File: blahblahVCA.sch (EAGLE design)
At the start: 29 parts, among them IC1 CA3080D, IC2 RC4558D, IC3 CA3130D, Q1 BCM847DS

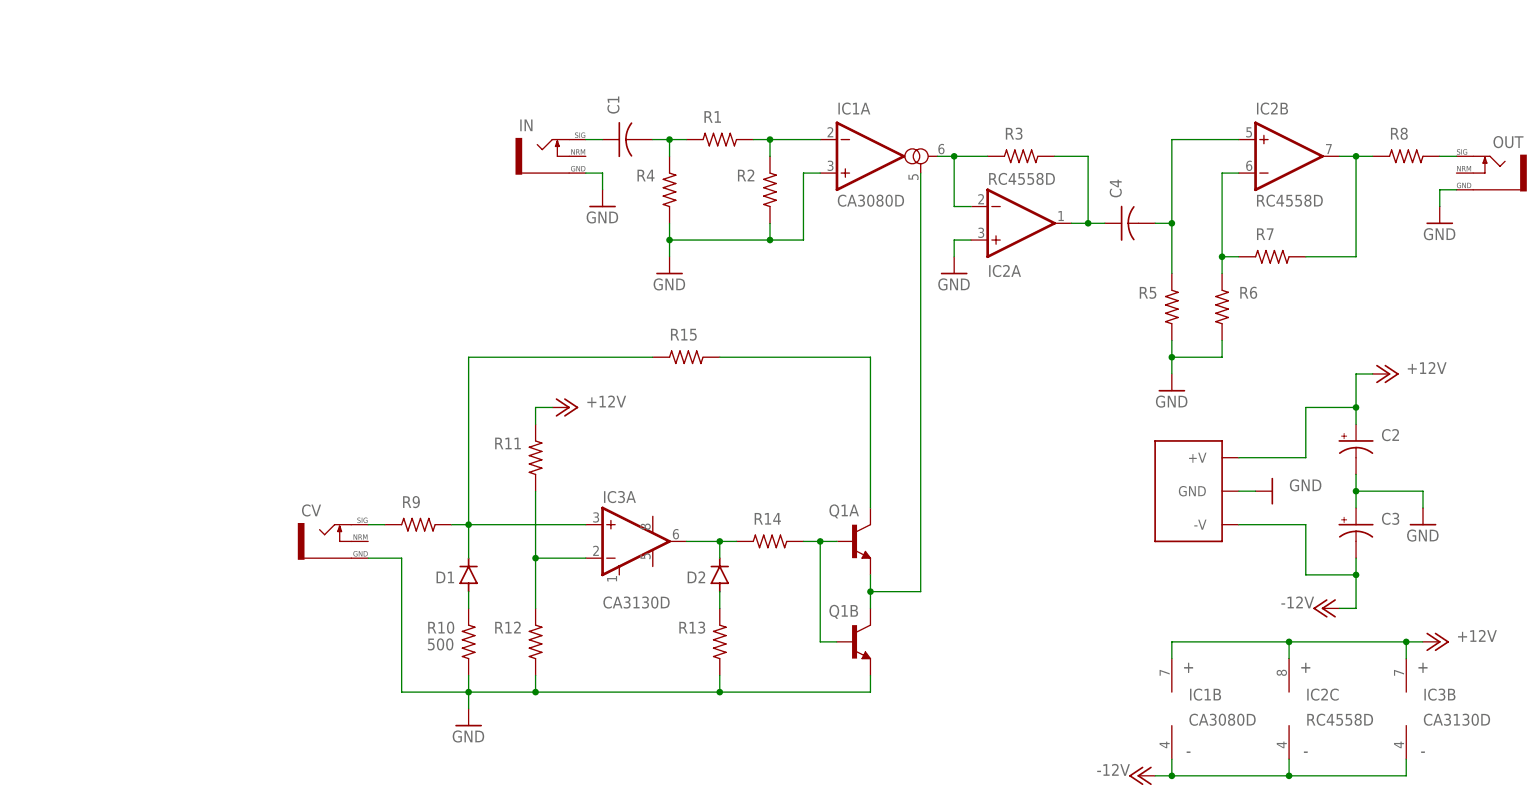
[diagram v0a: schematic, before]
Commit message: Add files via upload
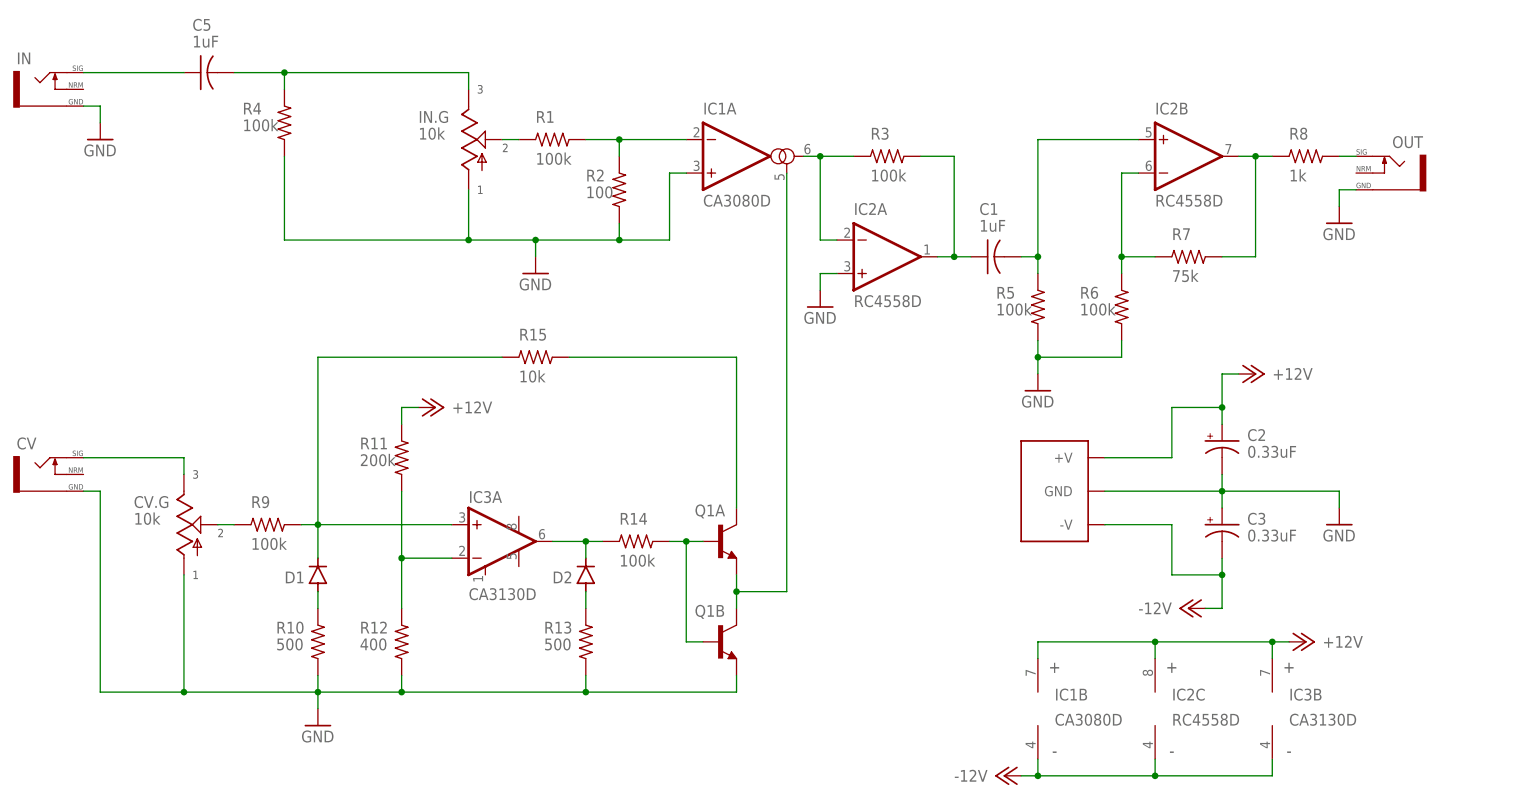
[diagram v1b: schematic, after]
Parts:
- removed C4: (no value), wb-rcl:C-05
- added C5: 1uF, wb-rcl:C-05
- added CV.G, IN.G: 10k, wb-potswitch:PALPHA
- C1: value (none) -> 1uF
- C2, C3: value (none) -> 0.33uF
- R1, R14, R3, R4, R5, R6, R9: value (none) -> 100k
- R11: value (none) -> 200k
- R12: value (none) -> 400
- R13: value (none) -> 500
- R15: value (none) -> 10k
- R2: value (none) -> 100
- R7: value (none) -> 75k
- R8: value (none) -> 1k
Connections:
- removed net N$1: C1.1, IN.TIP-SIG
- new net N$19: C5.1, IN.TIP-SIG
- new net N$20: C5.2, IN.G.3, R4.2
- new net N$21: CV.G.3, CV.TIP-SIG
- net GND: now also CV.G.1, IN.G.1, R6.1; no longer R6.2
- net N$10: now also CV.G.2; no longer CV.TIP-SIG
- net N$3: now also C1.1; no longer C4.1
- net N$5: now also IN.G.2; no longer C1.2, R4.2
- net N$6: now also C1.2; no longer C4.2
- net N$7: now also R6.2; no longer R6.1
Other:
- moved on the sheet: C1, C2, C3, CV, D1, D2, IC1A, IC1B, IC2A, IC2B, IC2C, IC3A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
